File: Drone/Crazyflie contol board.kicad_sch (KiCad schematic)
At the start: 27 parts, among them J1 Conn_01x05_Pin, J4 Conn_01x08_Pin, J5 Conn_01x04_Pin, P1 USB_C_Plug_USB2.0, SW1 SW_Push, SW2 SW_Push, SW3 SW_Push, SW4 SW_Push, SW5 SW_Push, SW6 SW_Push, SW7 SW_Push, SW8 SW_Push, U1 ESP32-S3-WROOM-1, U4 TPS63000, U5 NUF2221-Crazyflie-contol-boar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

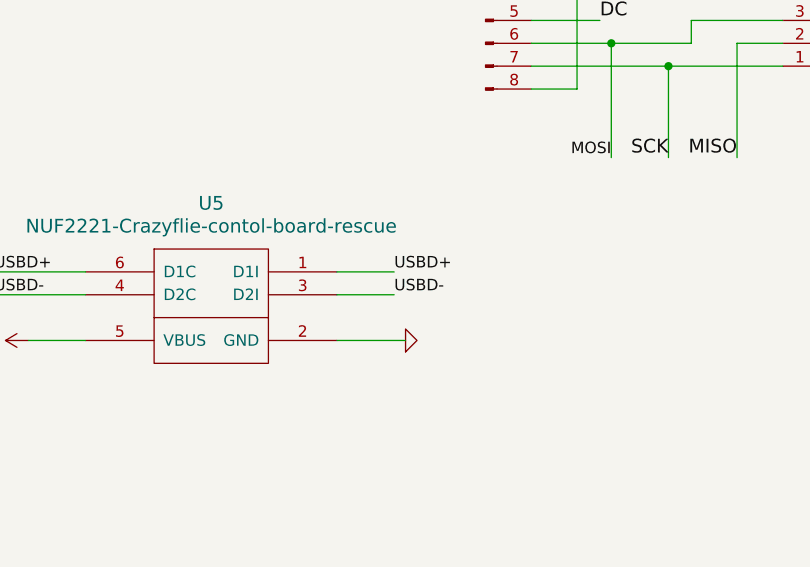
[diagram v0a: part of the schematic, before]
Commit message: save
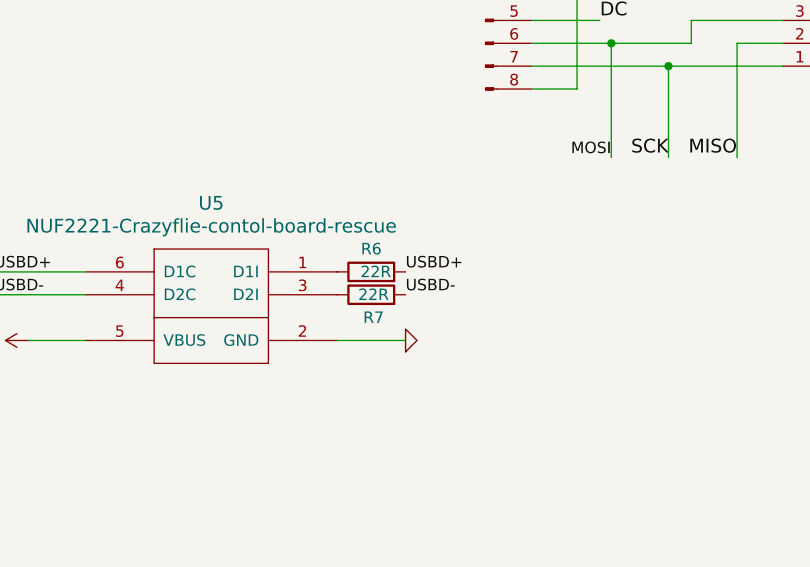
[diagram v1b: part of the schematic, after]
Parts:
- added R6, R7: 22R, Resistor_SMD:R_0603_1608Metric, symbol Device:R
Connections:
- net USBD+: now also R6.2; no longer U5.1 (D1I)
- net USBD-: now also R7.2; no longer U5.3 (D2I)
- new net: R7.1, U5.3 (D2I)
- new net: R6.1, U5.1 (D1I)
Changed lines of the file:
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@@
 	(wire
 		(pts
-			(xy 163.83 129.54) (xy 170.18 129.54)
-		)
-		(stroke
-			(width 0)
-			(type default)
-		)
-	)
-	(wire
-		(pts
 			(xy 242.57 74.93) (xy 247.65 74.93)
 		)
@@
 	(wire
 		(pts
-			(xy 163.83 132.08) (xy 170.18 132.08)
-		)
-		(stroke
-			(width 0)
-			(type default)
-		)
-	)
-	(wire
-		(pts
 			(xy 77.47 64.77) (xy 77.47 54.61)
 		)
@@
 	)
 	(label "USBD-"
-		(at 170.18 132.08 0)
+		(at 171.45 132.08 0)
 		(effects
 			(font
@@
 	)
 	(label "USBD+"
-		(at 170.18 129.54 0)
+		(at 171.45 129.54 0)
 		(effects
 			(font
@@
 	)
 	(symbol
+		(lib_id "Device:R")
+		(at 167.64 132.08 90)
+		(unit 1)
+		(exclude_from_sim no)
+		(in_bom yes)
+		(on_board yes)
+		(dnp no)
+		(property "Reference" "R7"
+			(at 167.894 134.62 90)
+			(effects
+				(font
+					(size 1.27 1.27)
+				)
+			)
+		)
+		(property "Value" "22R"
+			(at 167.894 132.08 90)
+			(effects
+				(font
+					(size 1.27 1.27)
+				)
+			)
+		)
+		(property "Footprint" "Resistor_SMD:R_0603_1608Metric"
+			(at 167.64 133.858 90)
+			(effects
+				(font
+					(size 1.27 1.27)
+				)
+				(hide yes)
+			)
+		)
+		(property "Datasheet" "~"
+			(at 167.64 132.08 0)
+			(effects
+				(font
+					(size 1.27 1.27)
+				)
+				(hide yes)
+			)
+		)
+		(property "Description" "Resistor"
+			(at 167.64 132.08 0)
+			(effects
+				(font
+					(size 1.27 1.27)
+				)
+				(hide yes)
+			)
+		)
+		(pin "2"
+		)
+		(pin "1"
+		)
+		(instances
+			(project ""
+				(path "/3e9fa01f-48e9-4c58-997e-0bab5b5694a8"
+					(reference "R7")
+					(unit 1)
+				)
+			)
+		)
+	)
+	(symbol
 		(lib_id "RF_Module:ESP32-S3-WROOM-1")
 		(at 140.97 55.88 0)
@@
 					(unit 1)
 				)
+			)
+		)
+	)
+	(symbol
+		(lib_id "Device:R")
+		(at 167.64 129.54 90)
+		(unit 1)
+		(exclude_from_sim no)
+		(in_bom yes)
+		(on_board yes)
+		(dnp no)
+		(property "Reference" "R6"
+			(at 167.64 127 90)
+			(effects
+				(font
+					(size 1.27 1.27)
+				)
+			)
+		)
+		(property "Value" "22R"
+			(at 168.148 129.54 90)
+			(effects
+				(font
+					(size 1.27 1.27)
+				)
+			)
+		)
+		(property "Footprint" "Resistor_SMD:R_0603_1608Metric"
+			(at 167.64 131.318 90)
+			(effects
+				(font
+					(size 1.27 1.27)
+				)
+				(hide yes)
+			)
+		)
+		(property "Datasheet" "~"
+			(at 167.64 129.54 0)
+			(effects
+				(font
+					(size 1.27 1.27)
+				)
+				(hide yes)
+			)
+		)
+		(property "Description" "Resistor"
+			(at 167.64 129.54 0)
+			(effects
+				(font
+					(size 1.27 1.27)
+				)
+				(hide yes)
+			)
+		)
+		(pin "2"
+		)
+		(pin "1"
+		)
+		(instances
+			(project ""
+				(path "/3e9fa01f-48e9-4c58-997e-0bab5b5694a8"
+					(reference "R6")
+					(unit 1)
+				)
